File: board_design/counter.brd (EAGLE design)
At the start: 54.3 x 94 mm, 24 parts, among them IC1 7805T

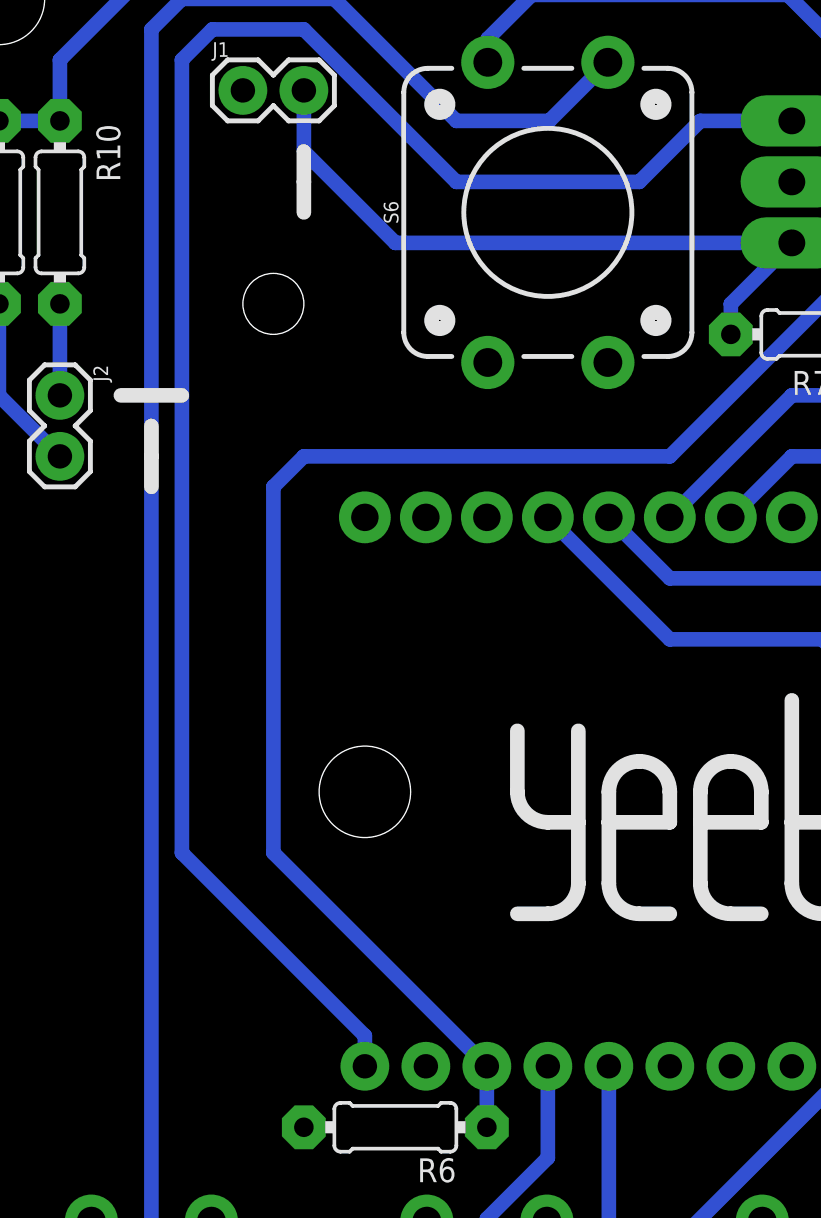
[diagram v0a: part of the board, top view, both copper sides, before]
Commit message: Board update
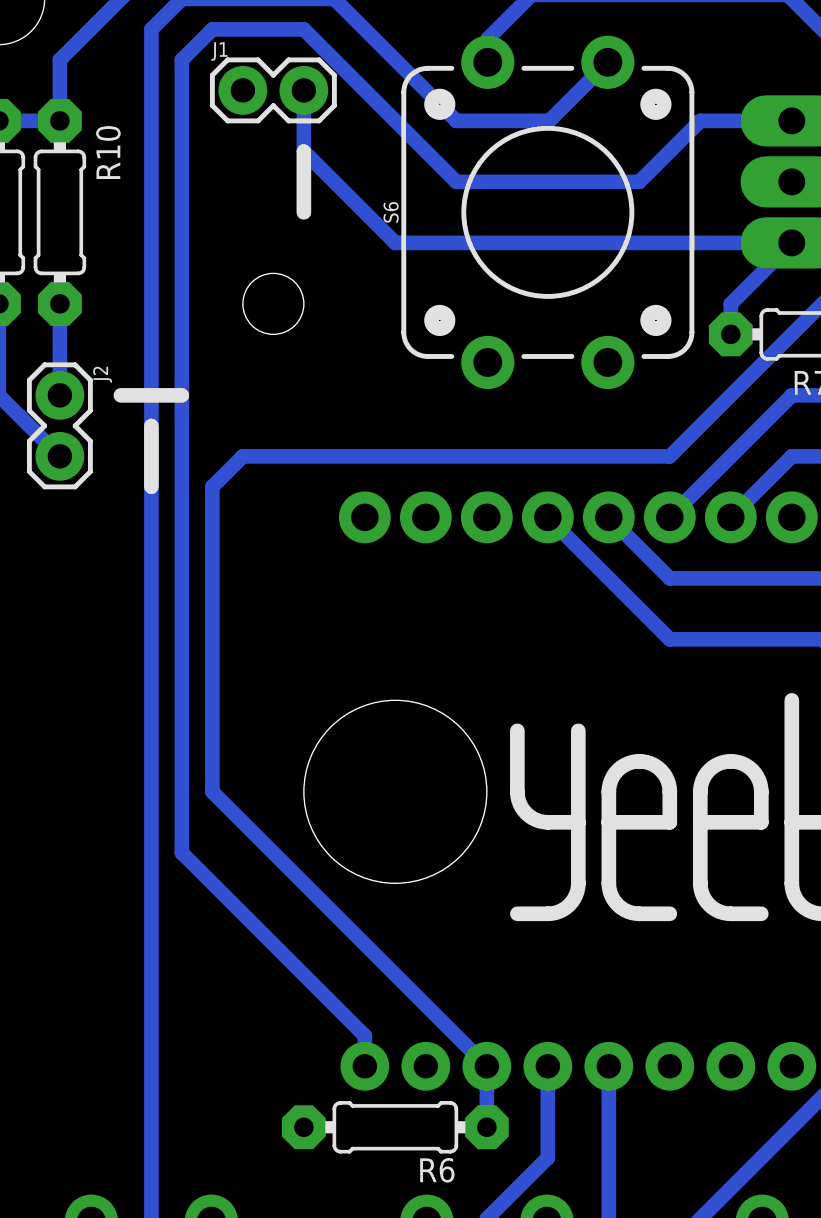
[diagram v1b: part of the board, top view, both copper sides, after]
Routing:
- net CLR: track 86.2 -> 89.8 mm
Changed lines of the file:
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@@
 <wire x1="54.28" y1="93.98" x2="0" y2="93.98" width="0" layer="20"/>
 <hole x="50.8" y="91.44" drill="3.81"/>
-<hole x="17.78" y="58.42" drill="3.81"/>
+<hole x="19.05" y="58.42" drill="7.62"/>
 <hole x="2.54" y="2.54" drill="3.81"/>
 <hole x="50.8" y="2.54" drill="3.81"/>
@@
 <wire x1="44.45" y1="27.94" x2="46.99" y2="27.94" width="0.6096" layer="25"/>
 <wire x1="7.62" y1="74.93" x2="10.16" y2="74.93" width="0.6096" layer="25"/>
-<wire x1="7.62" y1="72.39" x2="8.89" y2="72.39" width="0.6096" layer="26"/>
-<wire x1="8.89" y1="73.66" x2="8.89" y2="72.39" width="0.6096" layer="25"/>
-<wire x1="10.16" y1="72.39" x2="8.89" y2="72.39" width="0.6096" layer="26"/>
-<wire x1="8.89" y1="72.39" x2="8.89" y2="71.12" width="0.6096" layer="25"/>
+<wire x1="10.16" y1="72.39" x2="7.62" y2="72.39" width="0.6096" layer="26"/>
+<wire x1="8.89" y1="73.66" x2="8.89" y2="71.12" width="0.6096" layer="25"/>
 <wire x1="12.7" y1="85.09" x2="12.7" y2="82.55" width="0.6096" layer="26"/>
-<wire x1="13.97" y1="83.82" x2="15.24" y2="83.82" width="0.6096" layer="26"/>
-<wire x1="16.51" y1="83.82" x2="15.24" y2="83.82" width="0.6096" layer="26"/>
-<wire x1="15.24" y1="85.09" x2="15.24" y2="83.82" width="0.6096" layer="25"/>
-<wire x1="15.24" y1="83.82" x2="15.24" y2="82.55" width="0.6096" layer="25"/>
+<wire x1="16.51" y1="83.82" x2="13.97" y2="83.82" width="0.6096" layer="26"/>
+<wire x1="15.24" y1="85.09" x2="15.24" y2="82.55" width="0.6096" layer="25"/>
 </plain>
 <attributes>
@@
 <wire x1="39.37" y1="87.63" x2="39.37" y2="81.28" width="0.6096" layer="16"/>
 <wire x1="39.37" y1="81.28" x2="30.48" y2="72.39" width="0.6096" layer="16"/>
-<wire x1="30.48" y1="72.39" x2="15.24" y2="72.39" width="0.6096" layer="16"/>
-<wire x1="15.24" y1="72.39" x2="13.97" y2="71.12" width="0.6096" layer="16"/>
-<wire x1="13.97" y1="55.88" x2="22.86" y2="46.99" width="0.6096" layer="16"/>
-<wire x1="13.97" y1="71.12" x2="13.97" y2="55.88" width="0.6096" layer="16"/>
+<wire x1="30.48" y1="72.39" x2="12.7" y2="72.39" width="0.6096" layer="16"/>
+<wire x1="12.7" y1="72.39" x2="11.43" y2="71.12" width="0.6096" layer="16"/>
+<wire x1="11.43" y1="58.42" x2="22.86" y2="46.99" width="0.6096" layer="16"/>
+<wire x1="11.43" y1="71.12" x2="11.43" y2="58.42" width="0.6096" layer="16"/>
 <wire x1="22.86" y1="46.99" x2="22.86" y2="44.45" width="0.6096" layer="16"/>
 </signal>
